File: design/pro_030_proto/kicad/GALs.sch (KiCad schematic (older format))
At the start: 15 parts, among them IC2 ATF22V10C, IC3 ATF22V10C, IC4 ATF22V10C, IC5 ATF22V10C, IC6 ATF22V10C, IC7 ATF22V10C

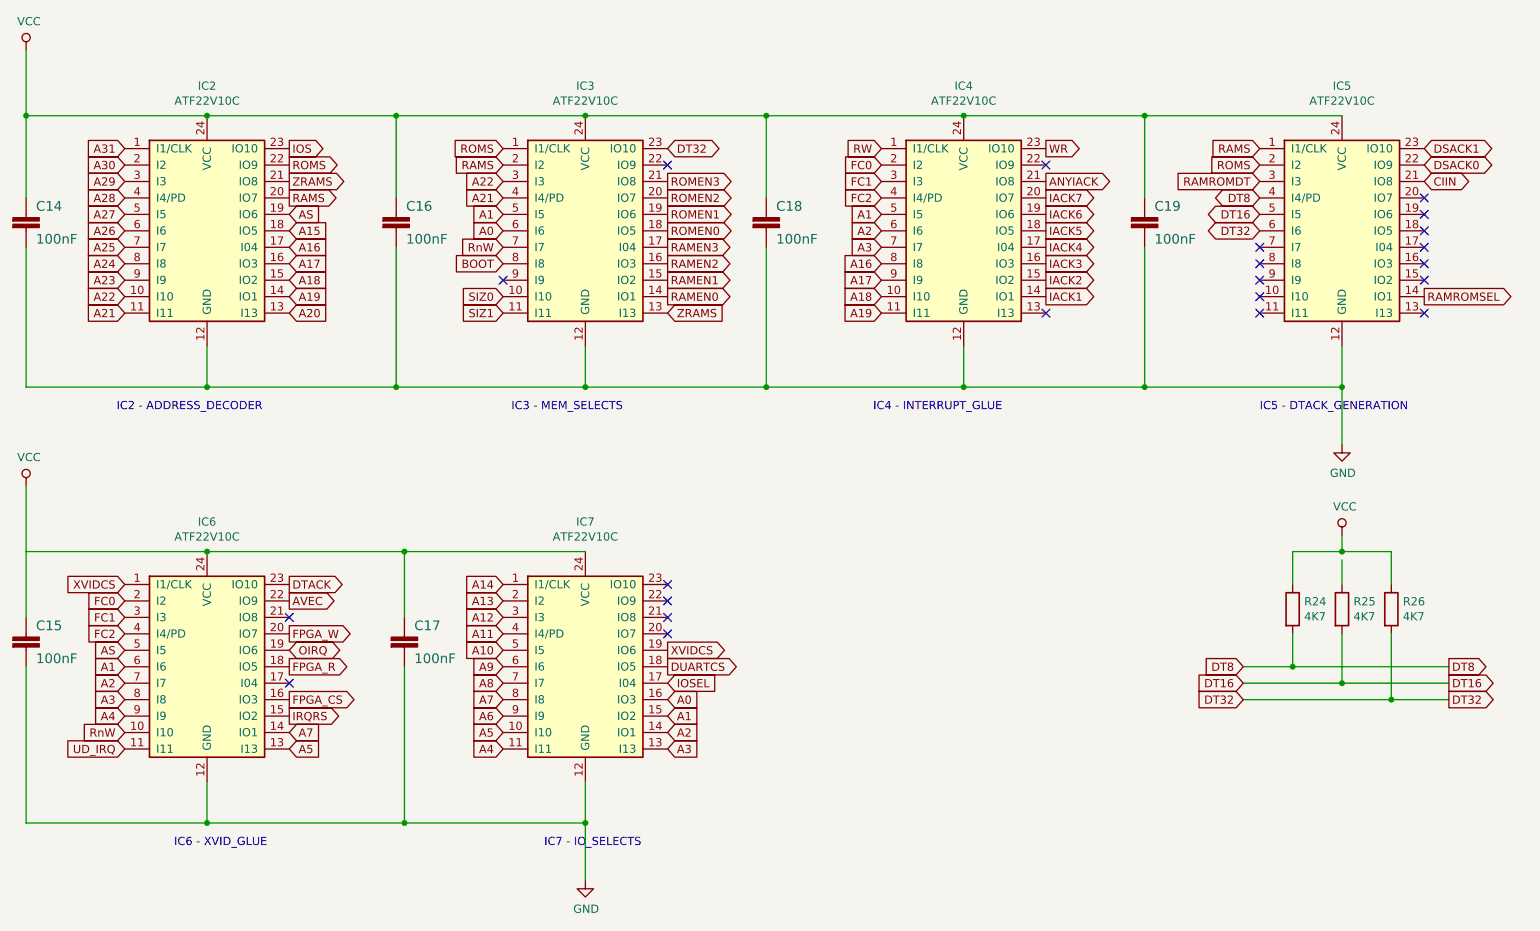
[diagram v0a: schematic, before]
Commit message: Finally fix ERC...
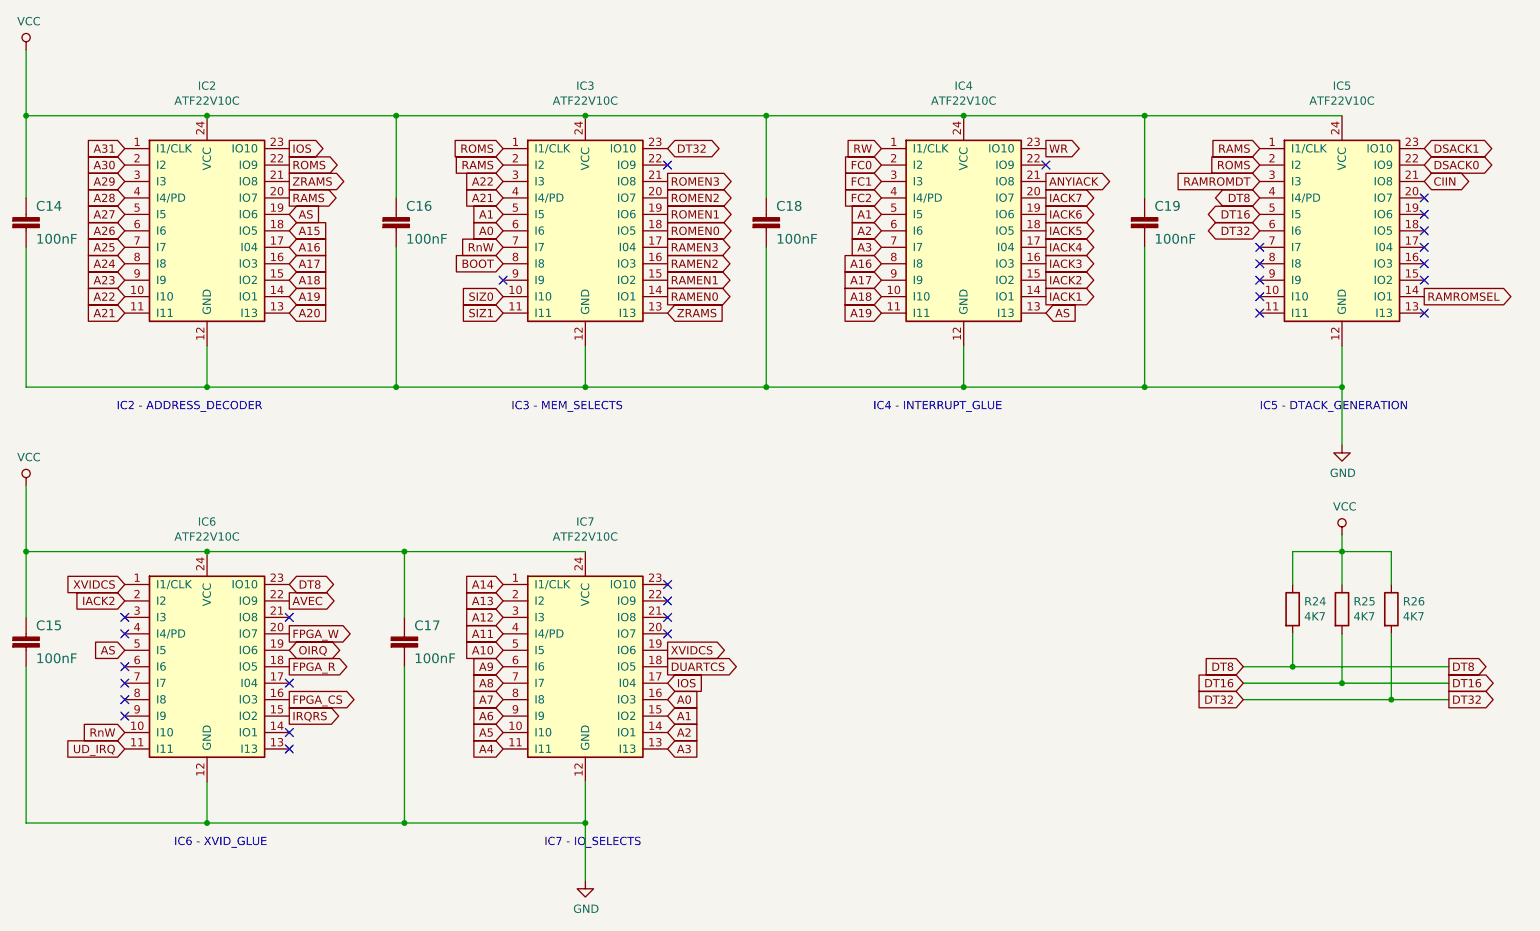
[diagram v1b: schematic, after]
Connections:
- net labels removed: DTACK, IOSEL
- wire segments 56 -> 57
- no-connect marks 22 -> 29
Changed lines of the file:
@@
 	4700 2950 4700 3200
-$Comp
-L power:GND #PWR032
-U 1 1 60F311F4
-P 9300 3550
-F 0 "#PWR032" H 9300 3300 50  0001 C CNN
-F 1 "GND" H 9305 3377 50  0000 C CNN
-F 2 "" H 9300 3550 50  0001 C CNN
-F 3 "" H 9300 3550 50  0001 C CNN
-	1    9300 3550
-	1    0    0    -1
-$EndComp
 $Comp
 L power:VCC #PWR029
@@
 Text GLabel 6500 1750 0    50   Input ~ 0
 RW
-Wire Wire Line
-	7000 3200 7000 2950
 $Comp
 L rosco_m68k:GAL22V10 IC4
@@
 	5800 1550 7000 1550
 Connection ~ 5800 1550
-Wire Wire Line
-	7000 3200 5800 3200
 Connection ~ 5800 3200
 Wire Wire Line
@@
 Connection ~ 7000 1550
 Connection ~ 8100 1550
-Wire Wire Line
-	7000 3200 8100 3200
-Connection ~ 7000 3200
 Connection ~ 8100 3200
 Wire Wire Line
@@
 Connection ~ 9300 4200
 Wire Wire Line
-	9300 4250 9300 4400
-Wire Wire Line
 	8700 4900 9000 4900
 Wire Wire Line
@@
 Text GLabel 1900 4400 0    50   Input ~ 0
 XVIDCS
-Text GLabel 2900 4400 2    50   Output ~ 0
-DTACK
+Text GLabel 2900 4400 2    50   3State ~ 0
+DT8
 Text GLabel 2900 4500 2    50   Output ~ 0
 AVEC
@@
 Text GLabel 1900 5300 0    50   Input ~ 0
 RnW
-Text GLabel 1900 4500 0    50   Input ~ 0
-FC0
-Text GLabel 1900 4600 0    50   Input ~ 0
-FC1
-Text GLabel 1900 4700 0    50   Input ~ 0
-FC2
 Text GLabel 1900 4800 0    50   Input ~ 0
 AS
@@
 	1    0    0    -1
 $EndComp
-Text GLabel 1900 4900 0    50   Input ~ 0
-A1
-Text GLabel 1900 5000 0    50   Input ~ 0
-A2
-Text GLabel 1900 5100 0    50   Input ~ 0
-A3
-Text GLabel 1900 5200 0    50   Input ~ 0
-A4
-Text GLabel 2900 5400 2    50   Input ~ 0
-A5
-Text GLabel 2900 5300 2    50   Input ~ 0
-A7
 Text GLabel 2900 5200 2    50   Output ~ 0
 IRQRS
@@
 	1    0    0    -1
 $EndComp
-Wire Wire Line
-	1300 3800 1300 4600
-Wire Wire Line
-	2400 4200 3600 4200
 $Comp
 L rosco_m68k-eagle-import:C2,5-3 C?
@@
 	1    0    0    -1
 $EndComp
-Wire Wire Line
-	3600 4600 3600 4200
-Connection ~ 3600 4200
-Wire Wire Line
-	3600 4200 4700 4200
 Wire Wire Line
 	3600 4900 3600 5850
@@
 A0
 Text GLabel 5200 5000 2    50   Input ~ 0
-IOSEL
+IOS
 Text GLabel 5200 4900 2    50   Output ~ 0
 DUARTCS
@@
 NoConn ~ 5200 4500
 NoConn ~ 5200 4400
-NoConn ~ 7500 2750
 Text GLabel 4200 2450 0    50   Input ~ 0
 BOOT
+Wire Wire Line
+	9300 4200 9300 4400
+Wire Wire Line
+	2400 4200 3600 4200
+Wire Wire Line
+	3600 4600 3600 4200
+Connection ~ 3600 4200
+Wire Wire Line
+	3600 4200 4700 4200
+Wire Wire Line
+	1300 3800 1300 4200
+Wire Wire Line
+	1300 4200 1300 4600
+Connection ~ 1300 4200
+Text GLabel 7500 2750 2    50   Input ~ 0
+AS
+Text GLabel 1900 4500 0    50   Input ~ 0
+IACK2
+NoConn ~ 1900 4600
+NoConn ~ 1900 4700
+NoConn ~ 1900 4900
+NoConn ~ 1900 5000
+NoConn ~ 1900 5100
+NoConn ~ 1900 5200
+NoConn ~ 2900 5300
+NoConn ~ 2900 5400
+Wire Wire Line
+	5800 3200 7000 3200
+Wire Wire Line
+	7000 2950 7000 3200
+Connection ~ 7000 3200
+Wire Wire Line
+	7000 3200 8100 3200
+$Comp
+L power:GND #PWR0102
+U 1 1 616CEF14
+P 9300 3550
+F 0 "#PWR0102" H 9300 3300 50  0001 C CNN
+F 1 "GND" H 9305 3377 50  0000 C CNN
+F 2 "" H 9300 3550 50  0001 C CNN
+F 3 "" H 9300 3550 50  0001 C CNN
+	1    9300 3550
+	1    0    0    -1
+$EndComp
 $EndSCHEMATC
